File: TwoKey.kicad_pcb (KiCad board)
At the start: 2 copper layers, 34 parts, among them J1 USB_C_Receptacle_USB2.0, SW1 SW_SPST, SW2 SW_SPST, SW3 BOOTSEL, SW4 RESET, U1 AMS1117-3.3, U2 W25Q128JVS, U3 RP2040TR7, X1 OSC

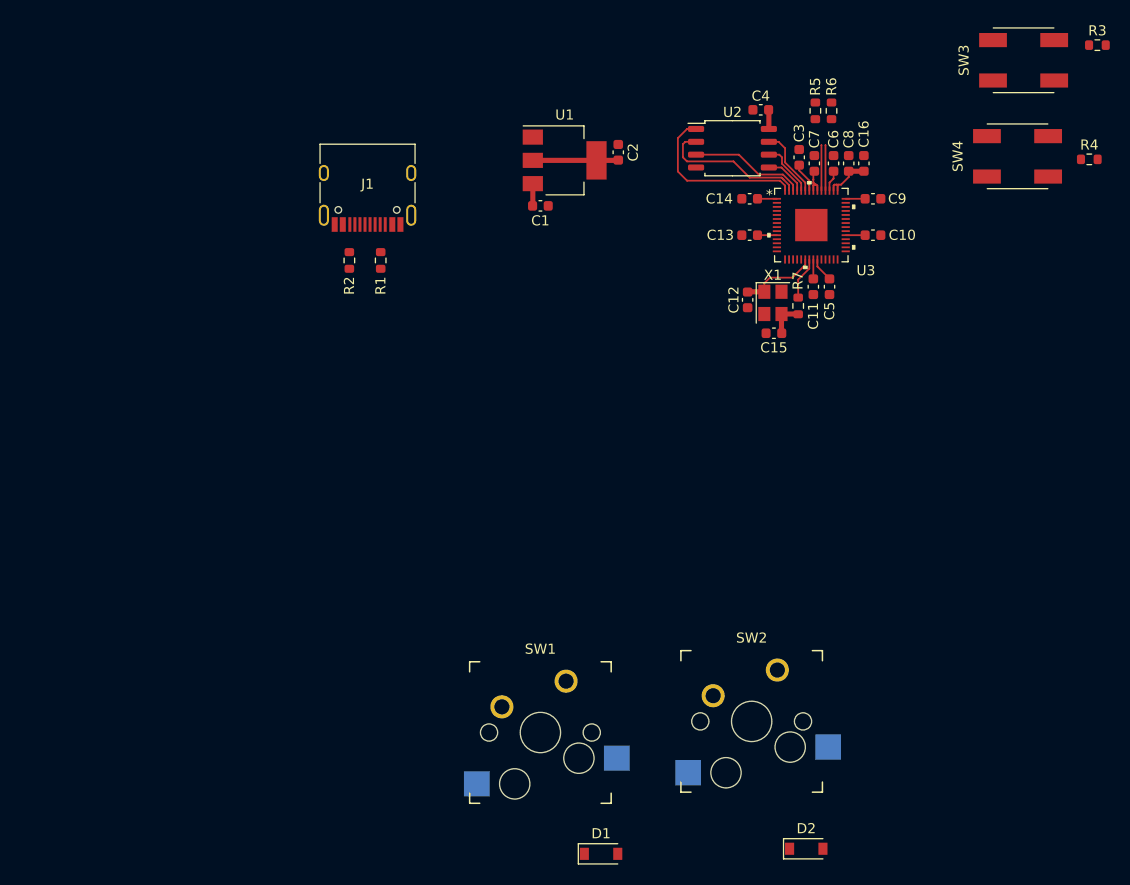
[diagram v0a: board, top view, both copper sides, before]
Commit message: Started work on condencing items
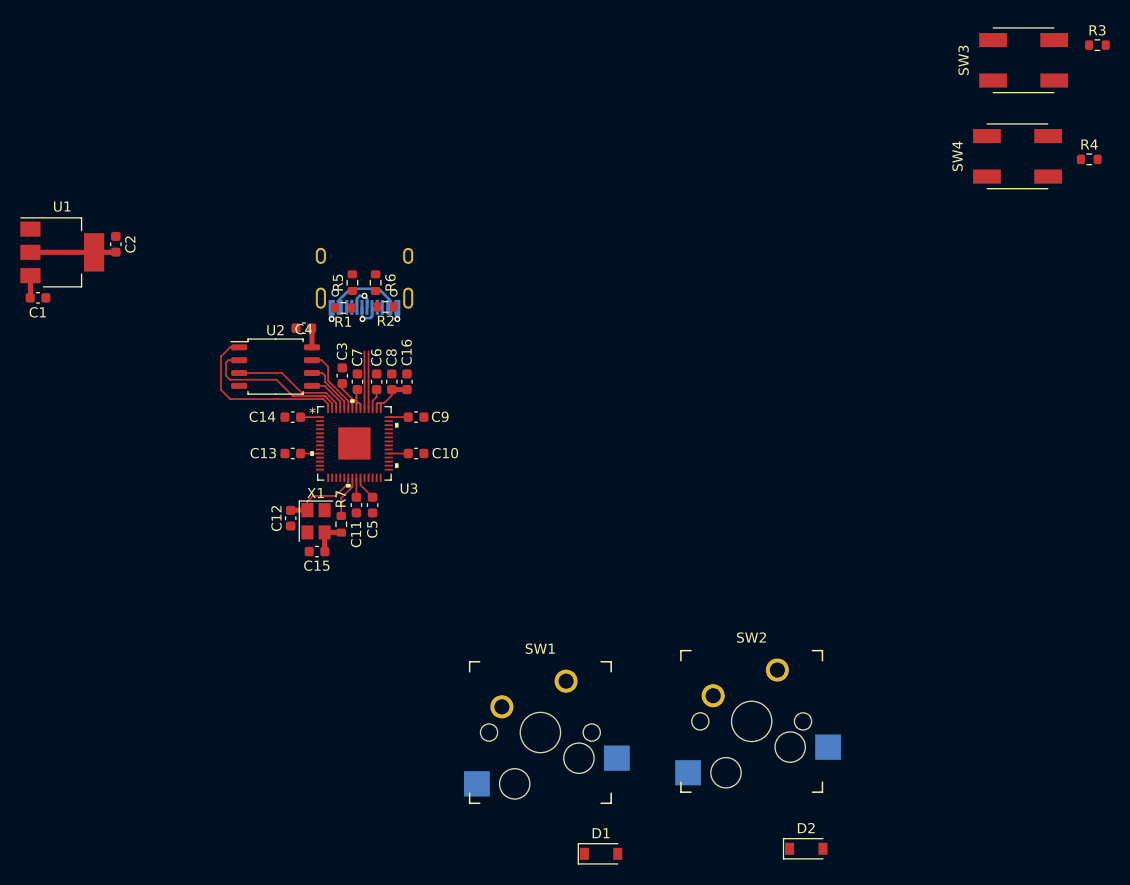
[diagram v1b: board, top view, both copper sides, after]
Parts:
- J1: moved to B.Cu
- moved C1 50.5 mm to (33.3, 43.0)
- moved C2 50.5 mm to (41.0, 37.7)
- moved U1 50.5 mm to (35.7, 38.5)
- moved C10 50.1 mm to (70.7, 58.4)
- moved C11 50.1 mm to (64.8, 63.5)
- moved C12 50.1 mm to (58.3, 64.8)
- moved C13 50.1 mm to (58.5, 58.4)
- moved C14 50.1 mm to (58.5, 54.8)
- moved C16 50.1 mm to (69.8, 51.3)
- moved C6 50.1 mm to (66.8, 51.3)
- moved C8 50.1 mm to (68.3, 51.3)
- moved C9 50.1 mm to (70.7, 54.8)
- moved R7 50.1 mm to (63.3, 65.4)
- moved U2 50.1 mm to (56.8, 49.8)
- moved U3 50.1 mm to (64.6, 57.4)
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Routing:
- net +5V: track 2.21 -> 9.57 mm
- net /USB_DN: track 0.00 -> 2.99 mm, vias 0 -> 1
- net /USB_DP: track 0.00 -> 2.91 mm, vias 0 -> 1
- net GND: track 0.00 -> 2.31 mm, vias 0 -> 2
- net Net-(R6-Pad1): track 4.50 -> 5.70 mm
- net Net-(R5-Pad1): track 4.50 -> 5.70 mm
